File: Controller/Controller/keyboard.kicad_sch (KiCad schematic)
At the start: 28 parts

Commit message: controller - changed resistor sizes
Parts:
- R1: footprint Resistor_THT:R_Axial_DIN0204_L3.6mm_D1.6mm_P5.08mm_Horizontal -> Resistor_THT:R_Axial_DIN0207_L6.3mm_D2.5mm_P7.62mm_Horizontal
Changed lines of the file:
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@@
       (effects (font (size 1.27 1.27)) (justify right))
     )
-    (property "Footprint" "Resistor_THT:R_Axial_DIN0204_L3.6mm_D1.6mm_P5.08mm_Horizontal" (at 65.278 44.45 90)
+    (property "Footprint" "Resistor_THT:R_Axial_DIN0207_L6.3mm_D2.5mm_P7.62mm_Horizontal" (at 65.278 44.45 90)
       (effects (font (size 1.27 1.27)) hide)
     )
@@
       (effects (font (size 1.27 1.27)) (justify right))
     )
-    (property "Footprint" "Resistor_THT:R_Axial_DIN0204_L3.6mm_D1.6mm_P5.08mm_Horizontal" (at 128.778 44.45 90)
+    (property "Footprint" "Resistor_THT:R_Axial_DIN0207_L6.3mm_D2.5mm_P7.62mm_Horizontal" (at 128.778 44.45 90)
       (effects (font (size 1.27 1.27)) hide)
     )
@@
       (effects (font (size 1.27 1.27)) (justify right))
     )
-    (property "Footprint" "Resistor_THT:R_Axial_DIN0204_L3.6mm_D1.6mm_P5.08mm_Horizontal" (at 52.578 95.25 90)
+    (property "Footprint" "Resistor_THT:R_Axial_DIN0207_L6.3mm_D2.5mm_P7.62mm_Horizontal" (at 52.578 95.25 90)
       (effects (font (size 1.27 1.27)) hide)
     )
@@
       (effects (font (size 1.27 1.27)) (justify right))
     )
-    (property "Footprint" "Resistor_THT:R_Axial_DIN0204_L3.6mm_D1.6mm_P5.08mm_Horizontal" (at 141.478 69.85 90)
+    (property "Footprint" "Resistor_THT:R_Axial_DIN0207_L6.3mm_D2.5mm_P7.62mm_Horizontal" (at 141.478 69.85 90)
       (effects (font (size 1.27 1.27)) hide)
     )
@@
       (effects (font (size 1.27 1.27)) (justify right))
     )
-    (property "Footprint" "Resistor_THT:R_Axial_DIN0204_L3.6mm_D1.6mm_P5.08mm_Horizontal" (at 141.478 44.45 90)
+    (property "Footprint" "Resistor_THT:R_Axial_DIN0207_L6.3mm_D2.5mm_P7.62mm_Horizontal" (at 141.478 44.45 90)
       (effects (font (size 1.27 1.27)) hide)
     )
@@
       (effects (font (size 1.27 1.27)) (justify right))
     )
-    (property "Footprint" "Resistor_THT:R_Axial_DIN0204_L3.6mm_D1.6mm_P5.08mm_Horizontal" (at 103.378 44.45 90)
+    (property "Footprint" "Resistor_THT:R_Axial_DIN0207_L6.3mm_D2.5mm_P7.62mm_Horizontal" (at 103.378 44.45 90)
       (effects (font (size 1.27 1.27)) hide)
     )
@@
       (effects (font (size 1.27 1.27)) (justify right))
     )
-    (property "Footprint" "Resistor_THT:R_Axial_DIN0204_L3.6mm_D1.6mm_P5.08mm_Horizontal" (at 77.978 95.25 90)
+    (property "Footprint" "Resistor_THT:R_Axial_DIN0207_L6.3mm_D2.5mm_P7.62mm_Horizontal" (at 77.978 95.25 90)
       (effects (font (size 1.27 1.27)) hide)
     )
@@
       (effects (font (size 1.27 1.27)) (justify right))
     )
-    (property "Footprint" "Resistor_THT:R_Axial_DIN0204_L3.6mm_D1.6mm_P5.08mm_Horizontal" (at 103.378 95.25 90)
+    (property "Footprint" "Resistor_THT:R_Axial_DIN0207_L6.3mm_D2.5mm_P7.62mm_Horizontal" (at 103.378 95.25 90)
       (effects (font (size 1.27 1.27)) hide)
     )
@@
       (effects (font (size 1.27 1.27)) (justify right))
     )
-    (property "Footprint" "Resistor_THT:R_Axial_DIN0204_L3.6mm_D1.6mm_P5.08mm_Horizontal" (at 154.178 69.85 90)
+    (property "Footprint" "Resistor_THT:R_Axial_DIN0207_L6.3mm_D2.5mm_P7.62mm_Horizontal" (at 154.178 69.85 90)
       (effects (font (size 1.27 1.27)) hide)
     )
@@
       (effects (font (size 1.27 1.27)) (justify right))
     )
-    (property "Footprint" "Resistor_THT:R_Axial_DIN0204_L3.6mm_D1.6mm_P5.08mm_Horizontal" (at 154.178 95.25 90)
+    (property "Footprint" "Resistor_THT:R_Axial_DIN0207_L6.3mm_D2.5mm_P7.62mm_Horizontal" (at 154.178 95.25 90)
       (effects (font (size 1.27 1.27)) hide)
     )
@@
       (effects (font (size 1.27 1.27)) (justify right))
     )
-    (property "Footprint" "Resistor_THT:R_Axial_DIN0204_L3.6mm_D1.6mm_P5.08mm_Horizontal" (at 52.578 69.85 90)
+    (property "Footprint" "Resistor_THT:R_Axial_DIN0207_L6.3mm_D2.5mm_P7.62mm_Horizontal" (at 52.578 69.85 90)
       (effects (font (size 1.27 1.27)) hide)
     )
@@
       (effects (font (size 1.27 1.27)) (justify right))
     )
-    (property "Footprint" "Resistor_THT:R_Axial_DIN0204_L3.6mm_D1.6mm_P5.08mm_Horizontal" (at 90.678 69.85 90)
+    (property "Footprint" "Resistor_THT:R_Axial_DIN0207_L6.3mm_D2.5mm_P7.62mm_Horizontal" (at 90.678 69.85 90)
       (effects (font (size 1.27 1.27)) hide)
     )
@@
       (effects (font (size 1.27 1.27)) (justify right))
     )
-    (property "Footprint" "Resistor_THT:R_Axial_DIN0204_L3.6mm_D1.6mm_P5.08mm_Horizontal" (at 90.678 95.25 90)
+    (property "Footprint" "Resistor_THT:R_Axial_DIN0207_L6.3mm_D2.5mm_P7.62mm_Horizontal" (at 90.678 95.25 90)
       (effects (font (size 1.27 1.27)) hide)
     )
@@
       (effects (font (size 1.27 1.27)) (justify right))
     )
-    (property "Footprint" "Resistor_THT:R_Axial_DIN0204_L3.6mm_D1.6mm_P5.08mm_Horizontal" (at 103.378 69.85 90)
+    (property "Footprint" "Resistor_THT:R_Axial_DIN0207_L6.3mm_D2.5mm_P7.62mm_Horizontal" (at 103.378 69.85 90)
       (effects (font (size 1.27 1.27)) hide)
     )
@@
       (effects (font (size 1.27 1.27)) (justify right))
     )
-    (property "Footprint" "Resistor_THT:R_Axial_DIN0204_L3.6mm_D1.6mm_P5.08mm_Horizontal" (at 90.678 44.45 90)
+    (property "Footprint" "Resistor_THT:R_Axial_DIN0207_L6.3mm_D2.5mm_P7.62mm_Horizontal" (at 90.678 44.45 90)
       (effects (font (size 1.27 1.27)) hide)
     )
@@
       (effects (font (size 1.27 1.27)) (justify right))
     )
-    (property "Footprint" "Resistor_THT:R_Axial_DIN0204_L3.6mm_D1.6mm_P5.08mm_Horizontal" (at 77.978 44.45 90)
+    (property "Footprint" "Resistor_THT:R_Axial_DIN0207_L6.3mm_D2.5mm_P7.62mm_Horizontal" (at 77.978 44.45 90)
       (effects (font (size 1.27 1.27)) hide)
     )
@@
       (effects (font (size 1.27 1.27)) (justify right))
     )
-    (property "Footprint" "Resistor_THT:R_Axial_DIN0204_L3.6mm_D1.6mm_P5.08mm_Horizontal" (at 166.878 95.25 90)
+    (property "Footprint" "Resistor_THT:R_Axial_DIN0207_L6.3mm_D2.5mm_P7.62mm_Horizontal" (at 166.878 95.25 90)
       (effects (font (size 1.27 1.27)) hide)
     )
@@
       (effects (font (size 1.27 1.27)) (justify right))
     )
-    (property "Footprint" "Resistor_THT:R_Axial_DIN0204_L3.6mm_D1.6mm_P5.08mm_Horizontal" (at 141.478 95.25 90)
+    (property "Footprint" "Resistor_THT:R_Axial_DIN0207_L6.3mm_D2.5mm_P7.62mm_Horizontal" (at 141.478 95.25 90)
       (effects (font (size 1.27 1.27)) hide)
     )
@@
       (effects (font (size 1.27 1.27)) (justify right))
     )
-    (property "Footprint" "Resistor_THT:R_Axial_DIN0204_L3.6mm_D1.6mm_P5.08mm_Horizontal" (at 154.178 44.45 90)
+    (property "Footprint" "Resistor_THT:R_Axial_DIN0207_L6.3mm_D2.5mm_P7.62mm_Horizontal" (at 154.178 44.45 90)
       (effects (font (size 1.27 1.27)) hide)
     )
@@
       (effects (font (size 1.27 1.27)) (justify right))
     )
-    (property "Footprint" "Resistor_THT:R_Axial_DIN0204_L3.6mm_D1.6mm_P5.08mm_Horizontal" (at 77.978 69.85 90)
+    (property "Footprint" "Resistor_THT:R_Axial_DIN0207_L6.3mm_D2.5mm_P7.62mm_Horizontal" (at 77.978 69.85 90)
       (effects (font (size 1.27 1.27)) hide)
     )
@@
       (effects (font (size 1.27 1.27)) (justify right))
     )
-    (property "Footprint" "Resistor_THT:R_Axial_DIN0204_L3.6mm_D1.6mm_P5.08mm_Horizontal" (at 65.278 69.85 90)
+    (property "Footprint" "Resistor_THT:R_Axial_DIN0207_L6.3mm_D2.5mm_P7.62mm_Horizontal" (at 65.278 69.85 90)
       (effects (font (size 1.27 1.27)) hide)
     )
@@
       (effects (font (size 1.27 1.27)) (justify right))
     )
-    (property "Footprint" "Resistor_THT:R_Axial_DIN0204_L3.6mm_D1.6mm_P5.08mm_Horizontal" (at 65.278 95.25 90)
+    (property "Footprint" "Resistor_THT:R_Axial_DIN0207_L6.3mm_D2.5mm_P7.62mm_Horizontal" (at 65.278 95.25 90)
       (effects (font (size 1.27 1.27)) hide)
     )
@@
       (effects (font (size 1.27 1.27)) (justify right))
     )
-    (property "Footprint" "Resistor_THT:R_Axial_DIN0204_L3.6mm_D1.6mm_P5.08mm_Horizontal" (at 116.078 95.25 90)
+    (property "Footprint" "Resistor_THT:R_Axial_DIN0207_L6.3mm_D2.5mm_P7.62mm_Horizontal" (at 116.078 95.25 90)
       (effects (font (size 1.27 1.27)) hide)
     )
@@
       (effects (font (size 1.27 1.27)) (justify right))
     )
-    (property "Footprint" "Resistor_THT:R_Axial_DIN0204_L3.6mm_D1.6mm_P5.08mm_Horizontal" (at 128.778 69.85 90)
+    (property "Footprint" "Resistor_THT:R_Axial_DIN0207_L6.3mm_D2.5mm_P7.62mm_Horizontal" (at 128.778 69.85 90)
       (effects (font (size 1.27 1.27)) hide)
     )
@@
       (effects (font (size 1.27 1.27)) (justify right))
     )
-    (property "Footprint" "Resistor_THT:R_Axial_DIN0204_L3.6mm_D1.6mm_P5.08mm_Horizontal" (at 116.078 69.85 90)
+    (property "Footprint" "Resistor_THT:R_Axial_DIN0207_L6.3mm_D2.5mm_P7.62mm_Horizontal" (at 116.078 69.85 90)
       (effects (font (size 1.27 1.27)) hide)
     )
@@
       (effects (font (size 1.27 1.27)) (justify right))
     )
-    (property "Footprint" "Resistor_THT:R_Axial_DIN0204_L3.6mm_D1.6mm_P5.08mm_Horizontal" (at 128.778 95.25 90)
+    (property "Footprint" "Resistor_THT:R_Axial_DIN0207_L6.3mm_D2.5mm_P7.62mm_Horizontal" (at 128.778 95.25 90)
       (effects (font (size 1.27 1.27)) hide)
     )
@@
       (effects (font (size 1.27 1.27)) (justify right))
     )
-    (property "Footprint" "Resistor_THT:R_Axial_DIN0204_L3.6mm_D1.6mm_P5.08mm_Horizontal" (at 52.578 44.45 90)
+    (property "Footprint" "Resistor_THT:R_Axial_DIN0207_L6.3mm_D2.5mm_P7.62mm_Horizontal" (at 52.578 44.45 90)
       (effects (font (size 1.27 1.27)) hide)
     )
@@
       (effects (font (size 1.27 1.27)) (justify right))
     )
-    (property "Footprint" "Resistor_THT:R_Axial_DIN0204_L3.6mm_D1.6mm_P5.08mm_Horizontal" (at 116.078 44.45 90)
-      (effects (font (size 1.27 1.27)) hide)
-    )
+    (property "Footprint" "Resistor_THT:R_Axial_DIN0207_L6.3mm_D2.5mm_P7.62mm_Horizontal" (at 116.078 44.45 90)
+      (effects (font (size 1.27 1.27)) hide)
+    )

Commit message: minor cleanup
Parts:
- R1: footprint Resistor_THT:R_Axial_DIN0207_L6.3mm_D2.5mm_P7.62mm_Horizontal -> Library:R_Axial_DIN0207_L6.3mm_D2.5mm_P7.62mm_Horizontal
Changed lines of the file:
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@@
       (effects (font (size 1.27 1.27)) (justify right))
     )
-    (property "Footprint" "Resistor_THT:R_Axial_DIN0207_L6.3mm_D2.5mm_P7.62mm_Horizontal" (at 65.278 44.45 90)
+    (property "Footprint" "Library:R_Axial_DIN0207_L6.3mm_D2.5mm_P7.62mm_Horizontal" (at 65.278 44.45 90)
       (effects (font (size 1.27 1.27)) hide)
     )
@@
       (effects (font (size 1.27 1.27)) (justify right))
     )
-    (property "Footprint" "Resistor_THT:R_Axial_DIN0207_L6.3mm_D2.5mm_P7.62mm_Horizontal" (at 128.778 44.45 90)
+    (property "Footprint" "Library:R_Axial_DIN0207_L6.3mm_D2.5mm_P7.62mm_Horizontal" (at 128.778 44.45 90)
       (effects (font (size 1.27 1.27)) hide)
     )
@@
       (effects (font (size 1.27 1.27)) (justify right))
     )
-    (property "Footprint" "Resistor_THT:R_Axial_DIN0207_L6.3mm_D2.5mm_P7.62mm_Horizontal" (at 52.578 95.25 90)
+    (property "Footprint" "Library:R_Axial_DIN0207_L6.3mm_D2.5mm_P7.62mm_Horizontal" (at 52.578 95.25 90)
       (effects (font (size 1.27 1.27)) hide)
     )
@@
       (effects (font (size 1.27 1.27)) (justify right))
     )
-    (property "Footprint" "Resistor_THT:R_Axial_DIN0207_L6.3mm_D2.5mm_P7.62mm_Horizontal" (at 141.478 69.85 90)
+    (property "Footprint" "Library:R_Axial_DIN0207_L6.3mm_D2.5mm_P7.62mm_Horizontal" (at 141.478 69.85 90)
       (effects (font (size 1.27 1.27)) hide)
     )
@@
       (effects (font (size 1.27 1.27)) (justify right))
     )
-    (property "Footprint" "Resistor_THT:R_Axial_DIN0207_L6.3mm_D2.5mm_P7.62mm_Horizontal" (at 141.478 44.45 90)
+    (property "Footprint" "Library:R_Axial_DIN0207_L6.3mm_D2.5mm_P7.62mm_Horizontal" (at 141.478 44.45 90)
       (effects (font (size 1.27 1.27)) hide)
     )
@@
       (effects (font (size 1.27 1.27)) (justify right))
     )
-    (property "Footprint" "Resistor_THT:R_Axial_DIN0207_L6.3mm_D2.5mm_P7.62mm_Horizontal" (at 103.378 44.45 90)
+    (property "Footprint" "Library:R_Axial_DIN0207_L6.3mm_D2.5mm_P7.62mm_Horizontal" (at 103.378 44.45 90)
       (effects (font (size 1.27 1.27)) hide)
     )
@@
       (effects (font (size 1.27 1.27)) (justify right))
     )
-    (property "Footprint" "Resistor_THT:R_Axial_DIN0207_L6.3mm_D2.5mm_P7.62mm_Horizontal" (at 77.978 95.25 90)
+    (property "Footprint" "Library:R_Axial_DIN0207_L6.3mm_D2.5mm_P7.62mm_Horizontal" (at 77.978 95.25 90)
       (effects (font (size 1.27 1.27)) hide)
     )
@@
       (effects (font (size 1.27 1.27)) (justify right))
     )
-    (property "Footprint" "Resistor_THT:R_Axial_DIN0207_L6.3mm_D2.5mm_P7.62mm_Horizontal" (at 103.378 95.25 90)
+    (property "Footprint" "Library:R_Axial_DIN0207_L6.3mm_D2.5mm_P7.62mm_Horizontal" (at 103.378 95.25 90)
       (effects (font (size 1.27 1.27)) hide)
     )
@@
       (effects (font (size 1.27 1.27)) (justify right))
     )
-    (property "Footprint" "Resistor_THT:R_Axial_DIN0207_L6.3mm_D2.5mm_P7.62mm_Horizontal" (at 154.178 69.85 90)
+    (property "Footprint" "Library:R_Axial_DIN0207_L6.3mm_D2.5mm_P7.62mm_Horizontal" (at 154.178 69.85 90)
       (effects (font (size 1.27 1.27)) hide)
     )
@@
       (effects (font (size 1.27 1.27)) (justify right))
     )
-    (property "Footprint" "Resistor_THT:R_Axial_DIN0207_L6.3mm_D2.5mm_P7.62mm_Horizontal" (at 154.178 95.25 90)
+    (property "Footprint" "Library:R_Axial_DIN0207_L6.3mm_D2.5mm_P7.62mm_Horizontal" (at 154.178 95.25 90)
       (effects (font (size 1.27 1.27)) hide)
     )
@@
       (effects (font (size 1.27 1.27)) (justify right))
     )
-    (property "Footprint" "Resistor_THT:R_Axial_DIN0207_L6.3mm_D2.5mm_P7.62mm_Horizontal" (at 52.578 69.85 90)
+    (property "Footprint" "Library:R_Axial_DIN0207_L6.3mm_D2.5mm_P7.62mm_Horizontal" (at 52.578 69.85 90)
       (effects (font (size 1.27 1.27)) hide)
     )
@@
       (effects (font (size 1.27 1.27)) (justify right))
     )
-    (property "Footprint" "Resistor_THT:R_Axial_DIN0207_L6.3mm_D2.5mm_P7.62mm_Horizontal" (at 90.678 69.85 90)
+    (property "Footprint" "Library:R_Axial_DIN0207_L6.3mm_D2.5mm_P7.62mm_Horizontal" (at 90.678 69.85 90)
       (effects (font (size 1.27 1.27)) hide)
     )
@@
       (effects (font (size 1.27 1.27)) (justify right))
     )
-    (property "Footprint" "Resistor_THT:R_Axial_DIN0207_L6.3mm_D2.5mm_P7.62mm_Horizontal" (at 90.678 95.25 90)
+    (property "Footprint" "Library:R_Axial_DIN0207_L6.3mm_D2.5mm_P7.62mm_Horizontal" (at 90.678 95.25 90)
       (effects (font (size 1.27 1.27)) hide)
     )
@@
       (effects (font (size 1.27 1.27)) (justify right))
     )
-    (property "Footprint" "Resistor_THT:R_Axial_DIN0207_L6.3mm_D2.5mm_P7.62mm_Horizontal" (at 103.378 69.85 90)
+    (property "Footprint" "Library:R_Axial_DIN0207_L6.3mm_D2.5mm_P7.62mm_Horizontal" (at 103.378 69.85 90)
       (effects (font (size 1.27 1.27)) hide)
     )
@@
       (effects (font (size 1.27 1.27)) (justify right))
     )
-    (property "Footprint" "Resistor_THT:R_Axial_DIN0207_L6.3mm_D2.5mm_P7.62mm_Horizontal" (at 90.678 44.45 90)
+    (property "Footprint" "Library:R_Axial_DIN0207_L6.3mm_D2.5mm_P7.62mm_Horizontal" (at 90.678 44.45 90)
       (effects (font (size 1.27 1.27)) hide)
     )
@@
       (effects (font (size 1.27 1.27)) (justify right))
     )
-    (property "Footprint" "Resistor_THT:R_Axial_DIN0207_L6.3mm_D2.5mm_P7.62mm_Horizontal" (at 77.978 44.45 90)
+    (property "Footprint" "Library:R_Axial_DIN0207_L6.3mm_D2.5mm_P7.62mm_Horizontal" (at 77.978 44.45 90)
       (effects (font (size 1.27 1.27)) hide)
     )
@@
       (effects (font (size 1.27 1.27)) (justify right))
     )
-    (property "Footprint" "Resistor_THT:R_Axial_DIN0207_L6.3mm_D2.5mm_P7.62mm_Horizontal" (at 166.878 95.25 90)
+    (property "Footprint" "Library:R_Axial_DIN0207_L6.3mm_D2.5mm_P7.62mm_Horizontal" (at 166.878 95.25 90)
       (effects (font (size 1.27 1.27)) hide)
     )
@@
       (effects (font (size 1.27 1.27)) (justify right))
     )
-    (property "Footprint" "Resistor_THT:R_Axial_DIN0207_L6.3mm_D2.5mm_P7.62mm_Horizontal" (at 141.478 95.25 90)
+    (property "Footprint" "Library:R_Axial_DIN0207_L6.3mm_D2.5mm_P7.62mm_Horizontal" (at 141.478 95.25 90)
       (effects (font (size 1.27 1.27)) hide)
     )
@@
       (effects (font (size 1.27 1.27)) (justify right))
     )
-    (property "Footprint" "Resistor_THT:R_Axial_DIN0207_L6.3mm_D2.5mm_P7.62mm_Horizontal" (at 154.178 44.45 90)
+    (property "Footprint" "Library:R_Axial_DIN0207_L6.3mm_D2.5mm_P7.62mm_Horizontal" (at 154.178 44.45 90)
       (effects (font (size 1.27 1.27)) hide)
     )
@@
       (effects (font (size 1.27 1.27)) (justify right))
     )
-    (property "Footprint" "Resistor_THT:R_Axial_DIN0207_L6.3mm_D2.5mm_P7.62mm_Horizontal" (at 77.978 69.85 90)
+    (property "Footprint" "Library:R_Axial_DIN0207_L6.3mm_D2.5mm_P7.62mm_Horizontal" (at 77.978 69.85 90)
       (effects (font (size 1.27 1.27)) hide)
     )
@@
       (effects (font (size 1.27 1.27)) (justify right))
     )
-    (property "Footprint" "Resistor_THT:R_Axial_DIN0207_L6.3mm_D2.5mm_P7.62mm_Horizontal" (at 65.278 69.85 90)
+    (property "Footprint" "Library:R_Axial_DIN0207_L6.3mm_D2.5mm_P7.62mm_Horizontal" (at 65.278 69.85 90)
       (effects (font (size 1.27 1.27)) hide)
     )
@@
       (effects (font (size 1.27 1.27)) (justify right))
     )
-    (property "Footprint" "Resistor_THT:R_Axial_DIN0207_L6.3mm_D2.5mm_P7.62mm_Horizontal" (at 65.278 95.25 90)
+    (property "Footprint" "Library:R_Axial_DIN0207_L6.3mm_D2.5mm_P7.62mm_Horizontal" (at 65.278 95.25 90)
       (effects (font (size 1.27 1.27)) hide)
     )
@@
       (effects (font (size 1.27 1.27)) (justify right))
     )
-    (property "Footprint" "Resistor_THT:R_Axial_DIN0207_L6.3mm_D2.5mm_P7.62mm_Horizontal" (at 116.078 95.25 90)
+    (property "Footprint" "Library:R_Axial_DIN0207_L6.3mm_D2.5mm_P7.62mm_Horizontal" (at 116.078 95.25 90)
       (effects (font (size 1.27 1.27)) hide)
     )
@@
       (effects (font (size 1.27 1.27)) (justify right))
     )
-    (property "Footprint" "Resistor_THT:R_Axial_DIN0207_L6.3mm_D2.5mm_P7.62mm_Horizontal" (at 128.778 69.85 90)
+    (property "Footprint" "Library:R_Axial_DIN0207_L6.3mm_D2.5mm_P7.62mm_Horizontal" (at 128.778 69.85 90)
       (effects (font (size 1.27 1.27)) hide)
     )
@@
       (effects (font (size 1.27 1.27)) (justify right))
     )
-    (property "Footprint" "Resistor_THT:R_Axial_DIN0207_L6.3mm_D2.5mm_P7.62mm_Horizontal" (at 116.078 69.85 90)
+    (property "Footprint" "Library:R_Axial_DIN0207_L6.3mm_D2.5mm_P7.62mm_Horizontal" (at 116.078 69.85 90)
       (effects (font (size 1.27 1.27)) hide)
     )
@@
       (effects (font (size 1.27 1.27)) (justify right))
     )
-    (property "Footprint" "Resistor_THT:R_Axial_DIN0207_L6.3mm_D2.5mm_P7.62mm_Horizontal" (at 128.778 95.25 90)
+    (property "Footprint" "Library:R_Axial_DIN0207_L6.3mm_D2.5mm_P7.62mm_Horizontal" (at 128.778 95.25 90)
       (effects (font (size 1.27 1.27)) hide)
     )
@@
       (effects (font (size 1.27 1.27)) (justify right))
     )
-    (property "Footprint" "Resistor_THT:R_Axial_DIN0207_L6.3mm_D2.5mm_P7.62mm_Horizontal" (at 52.578 44.45 90)
+    (property "Footprint" "Library:R_Axial_DIN0207_L6.3mm_D2.5mm_P7.62mm_Horizontal" (at 52.578 44.45 90)
       (effects (font (size 1.27 1.27)) hide)
     )
@@
       (effects (font (size 1.27 1.27)) (justify right))
     )
-    (property "Footprint" "Resistor_THT:R_Axial_DIN0207_L6.3mm_D2.5mm_P7.62mm_Horizontal" (at 116.078 44.45 90)
-      (effects (font (size 1.27 1.27)) hide)
-    )
+    (property "Footprint" "Library:R_Axial_DIN0207_L6.3mm_D2.5mm_P7.62mm_Horizontal" (at 116.078 44.45 90)
+      (effects (font (size 1.27 1.27)) hide)
+    )

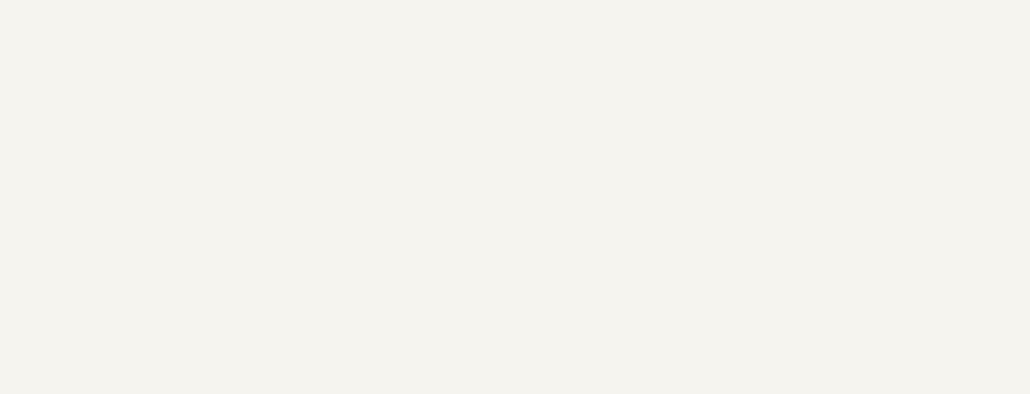
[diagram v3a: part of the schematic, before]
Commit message: Controller - incomplete fixes
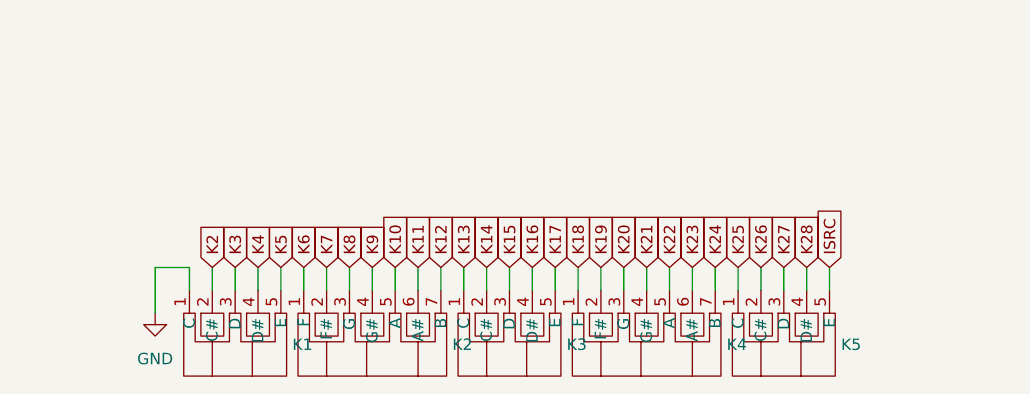
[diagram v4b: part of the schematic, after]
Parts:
- added K1, K3: ~, Library:Keyboard 5 keys, symbol Synth:Keyboard_5_keys
- added K2, K4: ~, symbol Synth:Keyboard_7_keys
- added K5: ~, symbol Synth:Keyboard_5_keys
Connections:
- net GND: now also K1.1 (C)
- net ISRC: now also K5.5 (E)
- net K10: now also K2.5 (A)
- net K11: now also K2.6 (A#)
- net K12: now also K2.7 (B)
- net K13: now also K3.1 (C)
- net K14: now also K3.2 (C#)
- net K15: now also K3.3 (D)
- net K16: now also K3.4 (D#)
- net K17: now also K3.5 (E)
- net K18: now also K4.1 (F)
- net K19: now also K4.2 (F#)
- net K2: now also K1.2 (C#)
- net K20: now also K4.3 (G)
- net K21: now also K4.4 (G#)
- net K22: now also K4.5 (A)
- net K23: now also K4.6 (A#)
- net K24: now also K4.7 (B)
- net K25: now also K5.1 (C)
- net K26: now also K5.2 (C#)
- net K27: now also K5.3 (D)
- net K28: now also K5.4 (D#)
- net K3: now also K1.3 (D)
- net K4: now also K1.4 (D#)
- net K5: now also K1.5 (E)
- net K6: now also K2.1 (F)
- net K7: now also K2.2 (F#)
- net K8: now also K2.3 (G)
- net K9: now also K2.4 (G#)
